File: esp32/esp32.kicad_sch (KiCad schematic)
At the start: 1 part, among them U1 ESP32-DEVKITC-32U

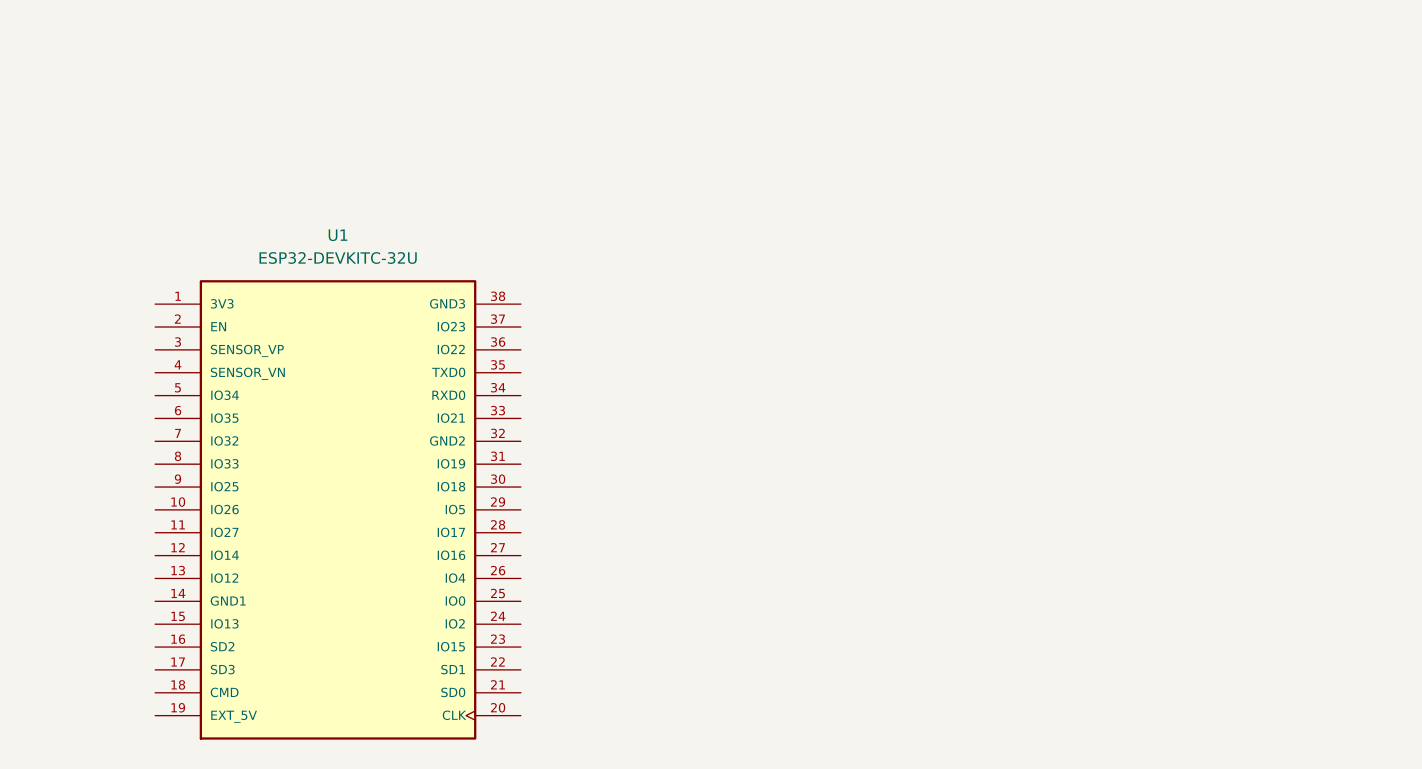
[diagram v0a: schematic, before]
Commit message: esp32
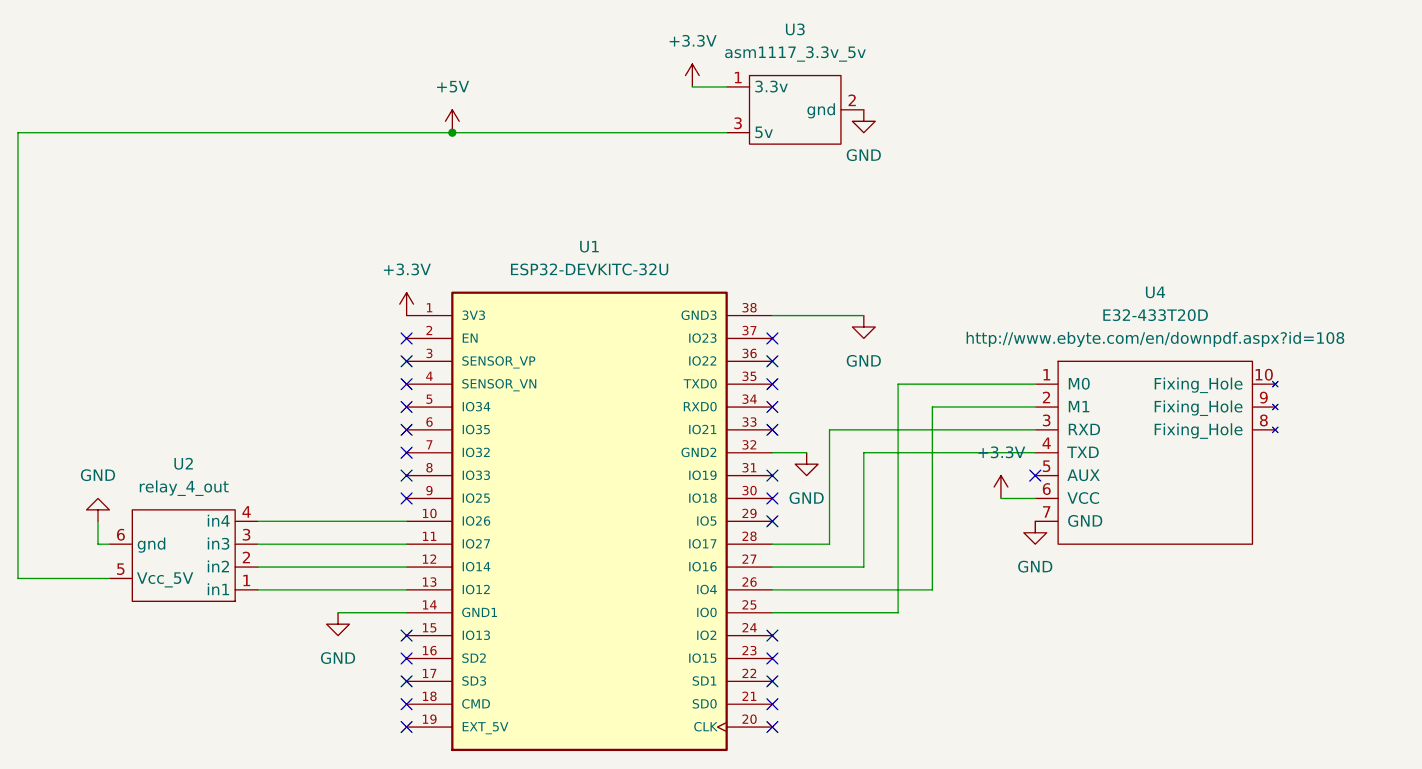
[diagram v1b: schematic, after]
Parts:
- added U2: relay_4_out, module_analog_sensor:relay_4_out, symbol module_analog_sensor:relay_4_out
- added U3: asm1117_3.3v_5v, module_analog_sensor:asm1117_3.3V_5V, symbol module_analog_sensor:asm1117_3.3v_5v
- added U4: E32-433T20D, 42CrMo4-KiCad-Library:E32-xxxT20D, symbol E32-xxxT20D:E32-433T20D
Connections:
- net +3.3V: now reaches U1.1 (3V3)
- net +3.3V: now also U3.1 (3.3v), U4.6 (VCC)
- net at U1.10 (IO26): now also U2.4 (in4)
- net at U1.11 (IO27): now also U2.3 (in3)
- net at U1.12 (IO14): now also U2.2 (in2)
- net at U1.13 (IO12): now also U2.1 (in1)
- net GND: now reaches U1.14 (GND1)
- net GND: now also U1.32 (GND2), U1.38 (GND3), U2.6 (gnd), U3.2 (gnd), U4.7 (GND)
- net at U1.25 (IO0): now also U4.1 (M0)
- net at U1.26 (IO4): now also U4.2 (M1)
- net at U1.27 (IO16): now also U4.4 (TXD)
- net at U1.28 (IO17): now also U4.3 (RXD)
- new net +5V: U2.5 (Vcc_5V), U3.3 (5v)
- no-connect marks 0 -> 27
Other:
- moved on the sheet: U1
